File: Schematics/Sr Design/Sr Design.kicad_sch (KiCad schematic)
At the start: 5 parts, among them J3 Barrel_Jack, J4 USB-A1HSW6

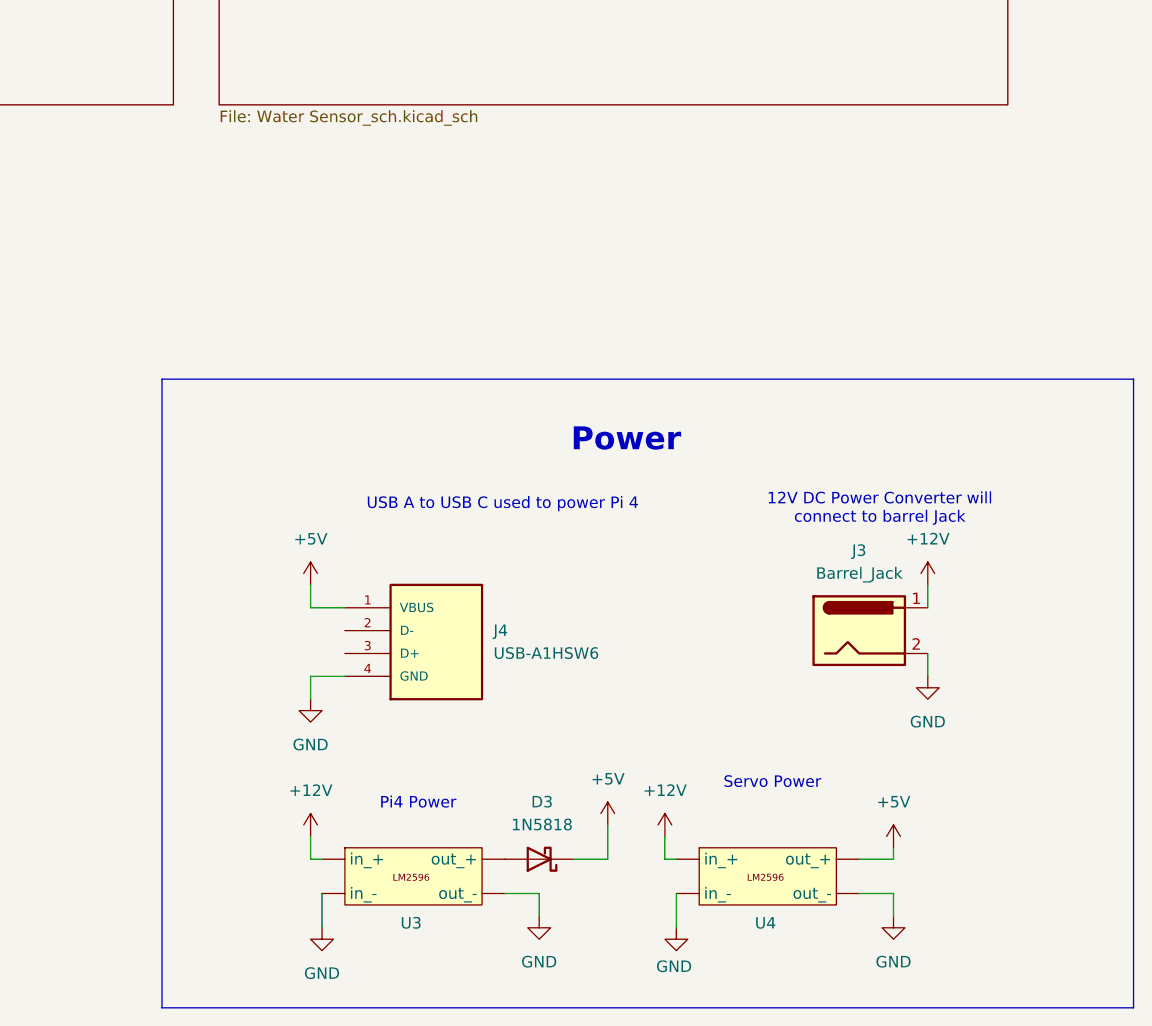
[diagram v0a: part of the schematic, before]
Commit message: scematics update
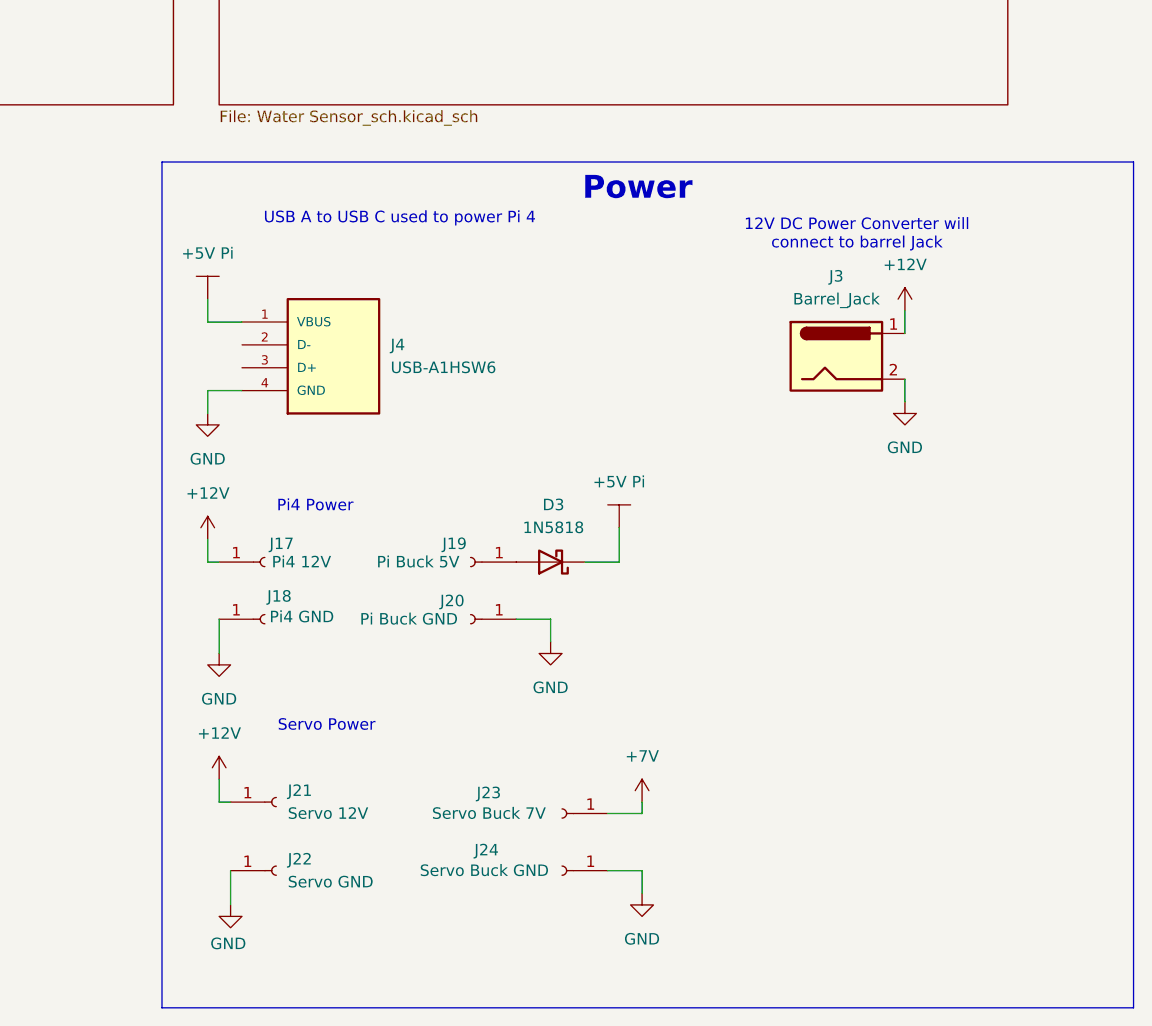
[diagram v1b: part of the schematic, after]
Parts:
- removed U3, U4: ~, symbol Turret_Power:_LM2596_Buck_Converter
- added J17: Pi4 12V, Connector_PinHeader_1.00mm:PinHeader_1x01_P1.00mm_Vertical, symbol Connector:Conn_01x01_Socket
- added J18: Pi4 GND, Connector_PinHeader_1.00mm:PinHeader_1x01_P1.00mm_Vertical, symbol Connector:Conn_01x01_Socket
- added J19: Pi Buck 5V, Connector_PinHeader_1.00mm:PinHeader_1x01_P1.00mm_Vertical, symbol Connector:Conn_01x01_Socket
- added J20: Pi Buck GND, Connector_PinHeader_1.00mm:PinHeader_1x01_P1.00mm_Vertical, symbol Connector:Conn_01x01_Socket
- added J21: Servo 12V, Connector_PinHeader_1.00mm:PinHeader_1x01_P1.00mm_Vertical, symbol Connector:Conn_01x01_Socket
- added J22: Servo GND, Connector_PinHeader_1.00mm:PinHeader_1x01_P1.00mm_Vertical, symbol Connector:Conn_01x01_Socket
- added J23: Servo Buck 7V, Connector_PinHeader_1.00mm:PinHeader_1x01_P1.00mm_Vertical, symbol Connector:Conn_01x01_Socket
- added J24: Servo Buck GND, Connector_PinHeader_1.00mm:PinHeader_1x01_P1.00mm_Vertical, symbol Connector:Conn_01x01_Socket
- J3: footprint (none) -> Connector_BarrelJack:BarrelJack_CUI_PJ-063AH_Horizontal
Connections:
- net +12V: now also J17.1 (Pin_1), J21.1 (Pin_1)
- net GND: now also J18.1 (Pin_1), J20.1 (Pin_1), J22.1 (Pin_1), J24.1 (Pin_1)
- net at D3.2 (A): now also J19.1 (Pin_1)
- net +5V renamed +5V Pi
- new net +7V: J23.1 (Pin_1)
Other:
- moved on the sheet: D3, J3, J4
